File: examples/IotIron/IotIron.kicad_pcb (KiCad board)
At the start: 2 copper layers, 100 x 36 mm, 93 parts

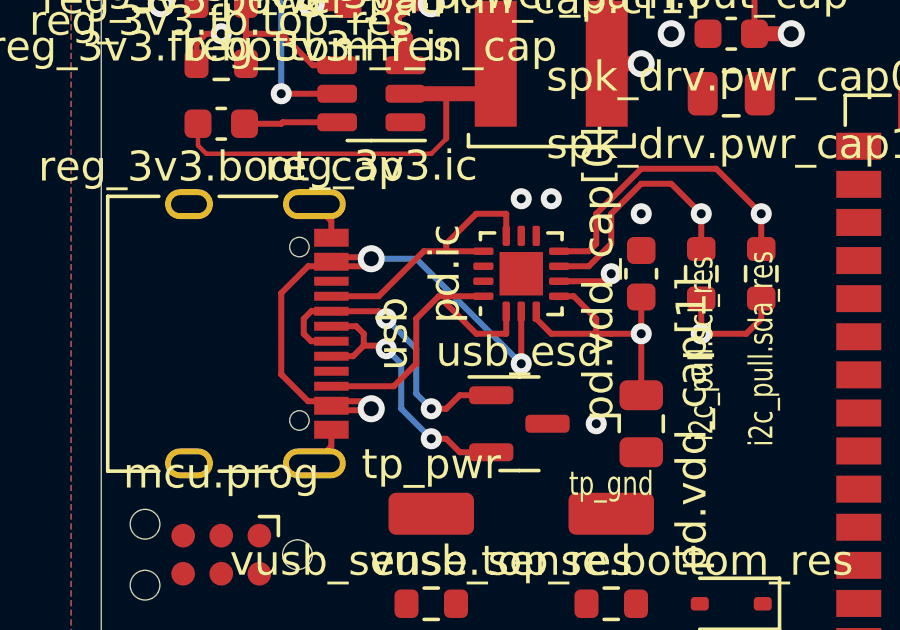
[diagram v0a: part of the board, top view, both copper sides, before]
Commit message: Update IotIron.kicad_pcb
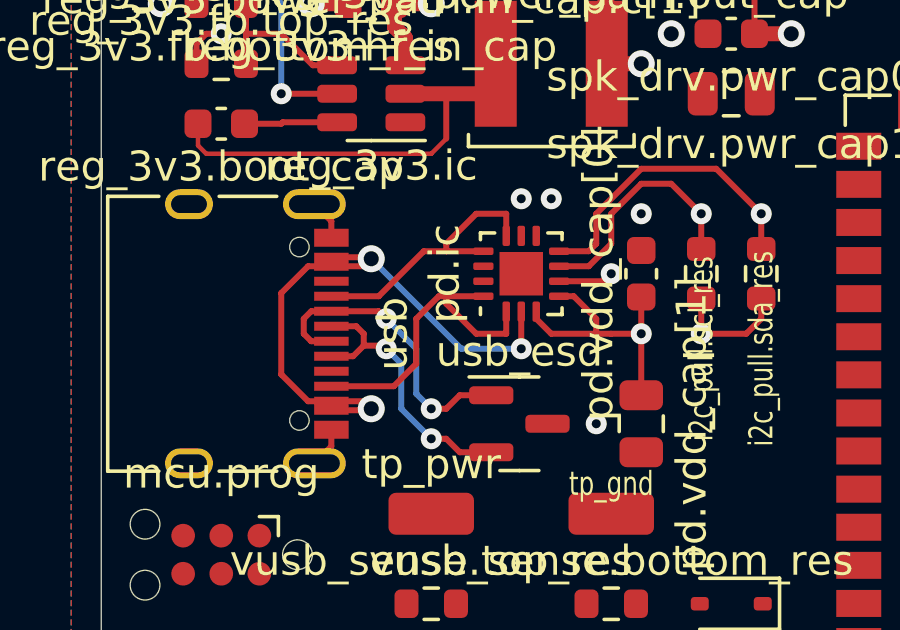
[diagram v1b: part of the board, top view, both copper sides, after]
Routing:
- net Ivusb: track 29.6 -> 28.9 mm
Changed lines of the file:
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@@
   (segment (start 193.5 76) (end 194.05 76) (width 0.5) (layer "F.Cu") (net 3))
   (segment (start 133.67 72.55) (end 134.95 72.55) (width 0.2) (layer "F.Cu") (net 3))
+  (segment (start 140 70.5) (end 140 69.2625) (width 0.2) (layer "F.Cu") (net 3))
   (segment (start 135.775 58.225) (end 135.775 59) (width 0.5) (layer "F.Cu") (net 3))
   (segment (start 133.67 67.45) (end 134.95 67.45) (width 0.2) (layer "F.Cu") (net 3))
@@
   (segment (start 134.95 72.55) (end 135 72.5) (width 0.2) (layer "F.Cu") (net 3))
   (segment (start 136.475 57.525) (end 135.775 58.225) (width 0.5) (layer "F.Cu") (net 3))
-  (segment (start 140 71) (end 140 69.2625) (width 0.2) (layer "F.Cu") (net 3))
   (segment (start 132.895 67.75) (end 133.67 67.75) (width 0.2) (layer "F.Cu") (net 3))
   (segment (start 135.775 59) (end 137 59) (width 0.5) (layer "F.Cu") (net 3))
@@
   (via (at 135 67.5) (size 0.9) (drill 0.5) (layers "F.Cu" "B.Cu") (net 3))
   (via (at 193 75.5) (size 0.7) (drill 0.3) (layers "F.Cu" "B.Cu") (net 3))
-  (via (at 140 71) (size 0.7) (drill 0.3) (layers "F.Cu" "B.Cu") (net 3))
+  (via (at 140 70.5) (size 0.7) (drill 0.3) (layers "F.Cu" "B.Cu") (net 3))
   (via (at 137.5 55.5) (size 0.9) (drill 0.5) (layers "F.Cu" "B.Cu") (net 3))
   (via (at 203 74.5) (size 0.9) (drill 0.5) (layers "F.Cu" "B.Cu") (net 3))
@@
   (via (at 132 57) (size 0.9) (drill 0.5) (layers "F.Cu" "B.Cu") (net 3))
   (via (at 135 72.5) (size 0.9) (drill 0.5) (layers "F.Cu" "B.Cu") (net 3))
-  (segment (start 136.5 67.5) (end 140 71) (width 0.2) (layer "B.Cu") (net 3))
-  (segment (start 135 67.5) (end 136.5 67.5) (width 0.2) (layer "B.Cu") (net 3))
+  (segment (start 138 70.5) (end 135 67.5) (width 0.2) (layer "B.Cu") (net 3))
+  (segment (start 140 70.5) (end 138 70.5) (width 0.2) (layer "B.Cu") (net 3))
   (segment (start 145.5625 56.25) (end 146.5 56.25) (width 0.2) (layer "F.Cu") (net 4))
   (segment (start 133.67 73.755) (end 133.67 73.35) (width 0.2) (layer "F.Cu") (net 4))
@@
       0d21ae96-2daa-474f-a3a7-d79d4792b5b2
       0ded325b-6ac3-49f7-8175-7a20026109cf
+      0f1ec1c9-dbf0-4d51-9b56-e5f23e76bb40
       11aa9a10-edfd-42d9-8035-eec5f5ac0ec1
       12299290-c0e5-4407-9de9-b31833e28f51
@@
       61eef90d-cc08-445c-b41c-5bb22086a5f0
       629b89a6-7f3b-43c3-a5cc-dad2f612e232
+      680c9fb0-26ab-4640-8bd3-d7b203450555
       6ab5854d-f830-4714-b2fa-0742e3bfd0fc
+      6be1ea21-7127-4e72-95b1-20e3b9ba4b75
       754fab17-a229-44a8-a0b7-2e60cb356246
       76b3256e-79bd-4915-92e3-67d793cf8f84
@@
       7a471fa2-cc53-41a3-abef-a48c5e686c82
       8422cfc1-f5bc-42f1-85ff-49716f3c9d26
-      86b3cff4-767e-4708-9fd5-11427b076157
       89668dc8-29ef-40c8-b578-6a3a4cd0354d
       89f0feab-c873-41a9-8a25-39d51095b8bf
